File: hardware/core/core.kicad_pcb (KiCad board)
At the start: 2 copper layers, 23 x 33.5 mm, 30 parts, among them J1 MOLEX_SlimStack_505550-1020, J2 Conn_01x02_Pin, U1 XIAO-NRF54L15, U2 BQ25173DSG, U3 BQ25570, U5 AXP1T34

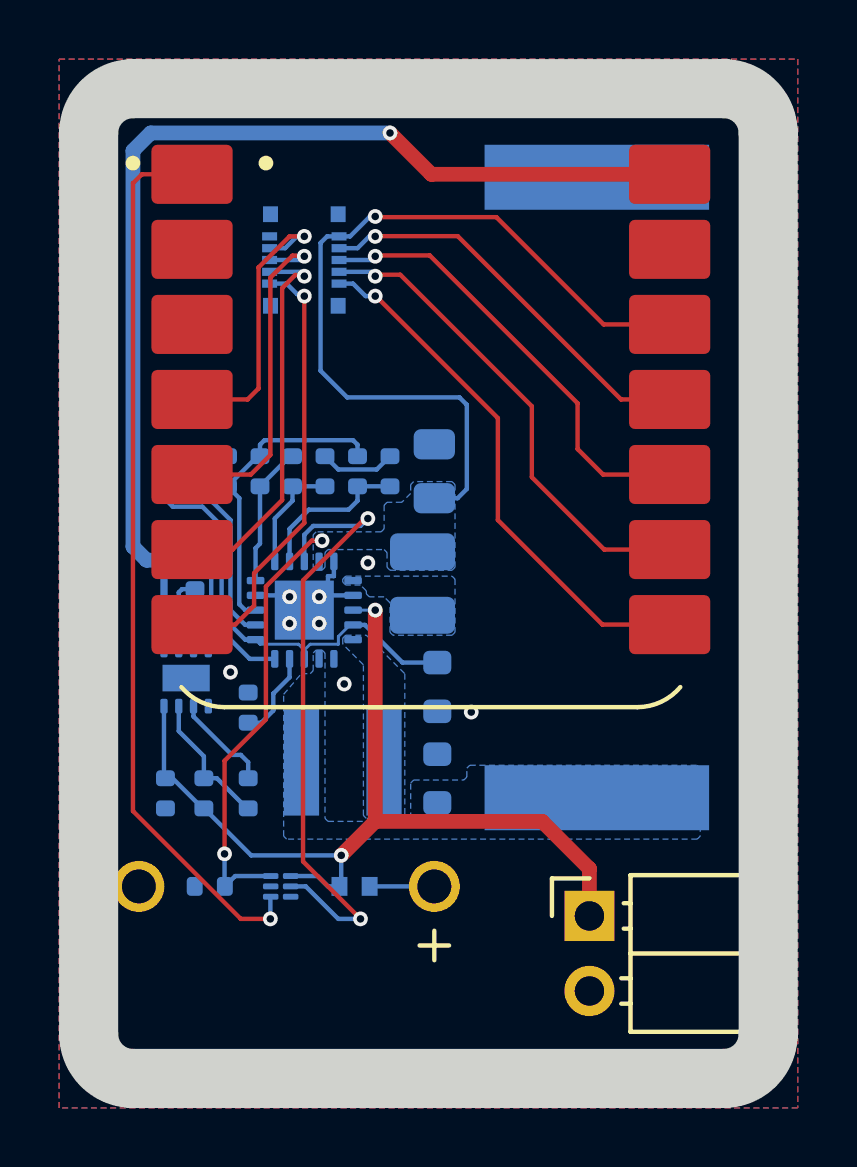
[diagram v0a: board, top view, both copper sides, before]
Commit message: bom updates
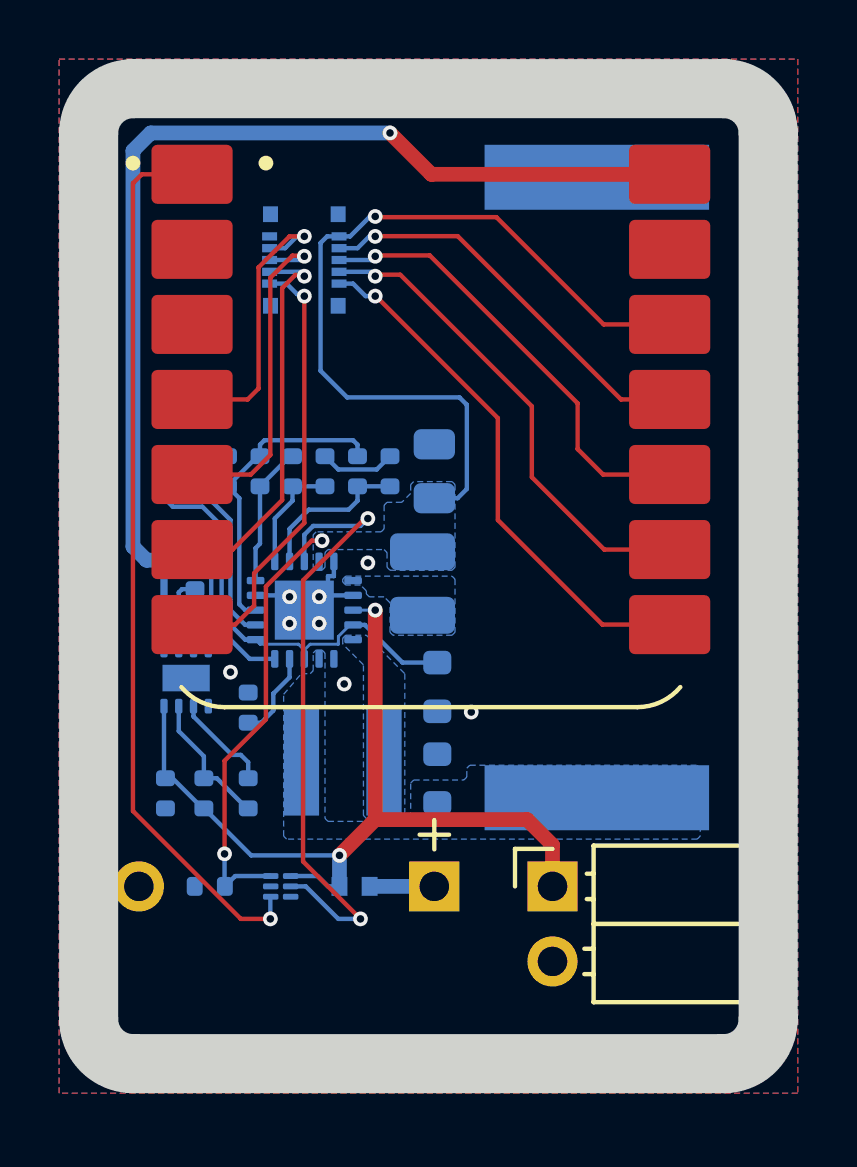
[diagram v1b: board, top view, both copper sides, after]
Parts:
- J2: footprint connectors:PinHeader_1x02_P2.54mm_Horizontal -> connectors:PD_801-83-002-20-001101
- moved Cb1 6.65 mm to (87.2, 77.0), turned to 0 degrees
- moved J2 1.60 mm to (94.6, 77.0)
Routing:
- net VCAP: track 31.4 -> 29.7 mm
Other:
- board size 23 x 33.5 mm -> 23 x 33 mm
- board text added: "${TITLE} V${REVISION}"
